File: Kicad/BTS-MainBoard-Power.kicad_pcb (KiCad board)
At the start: 2 copper layers, 101.6 x 95.3 mm, 47 parts, among them J1 +12VIn, J10 Conn_01x02, J11 Conn_01x02, J12 Conn_01x02, J13 Conn_01x02, J14 Conn_01x02, J15 Conn_01x02, J16 Conn_01x02, J17 Conn_01x02, J18 Conn_01x02, J19 Conn_01x02, J2 GNDIn, J3 Conn_01x14, J4 Conn_01x02, J5 Conn_01x02, J6 Conn_01x02, J7 Conn_01x02, J8 Conn_01x02, J9 Conn_01x02, Q1 STD80N6F6, Q2 STD80N6F6, Q3 STD80N6F6, Q4 STD80N6F6

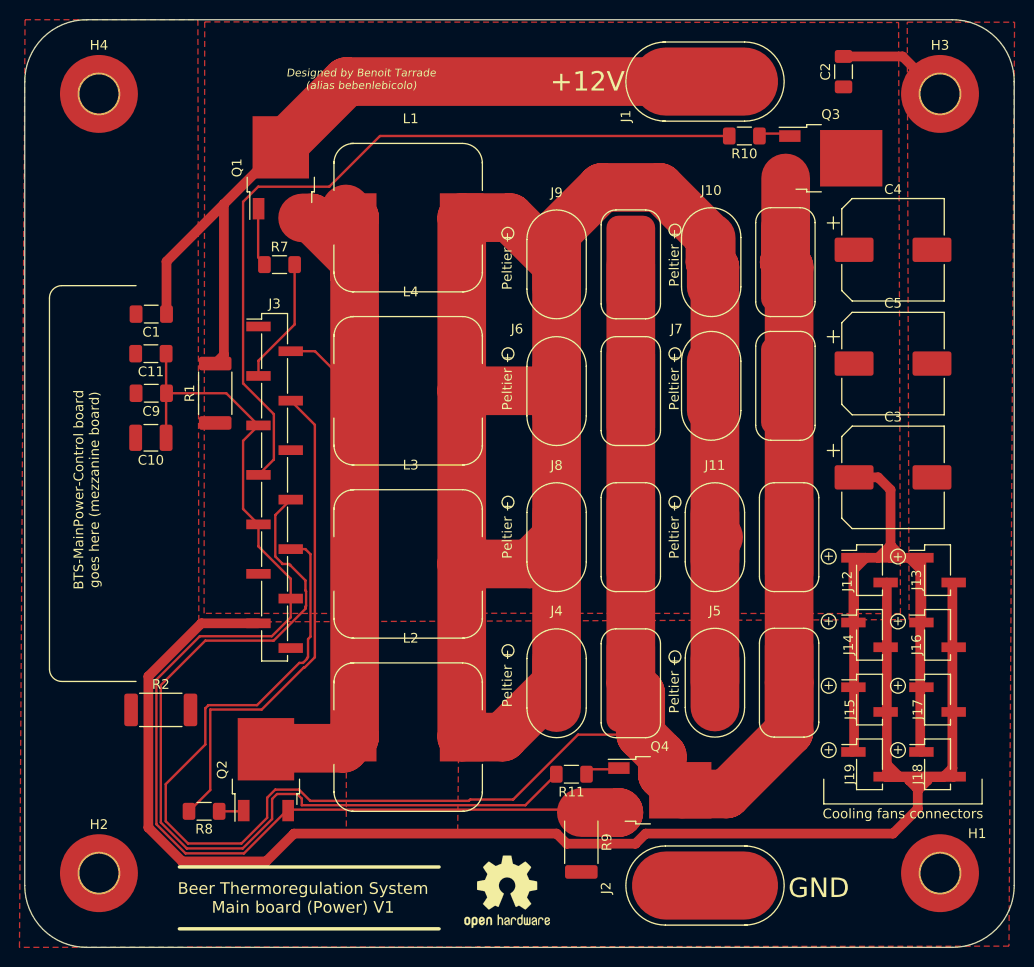
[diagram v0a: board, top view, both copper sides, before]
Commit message: Migrated kicad files to version 6
Signed-off-by: bebenlebricolo <benoittarrade@hotmail.fr>
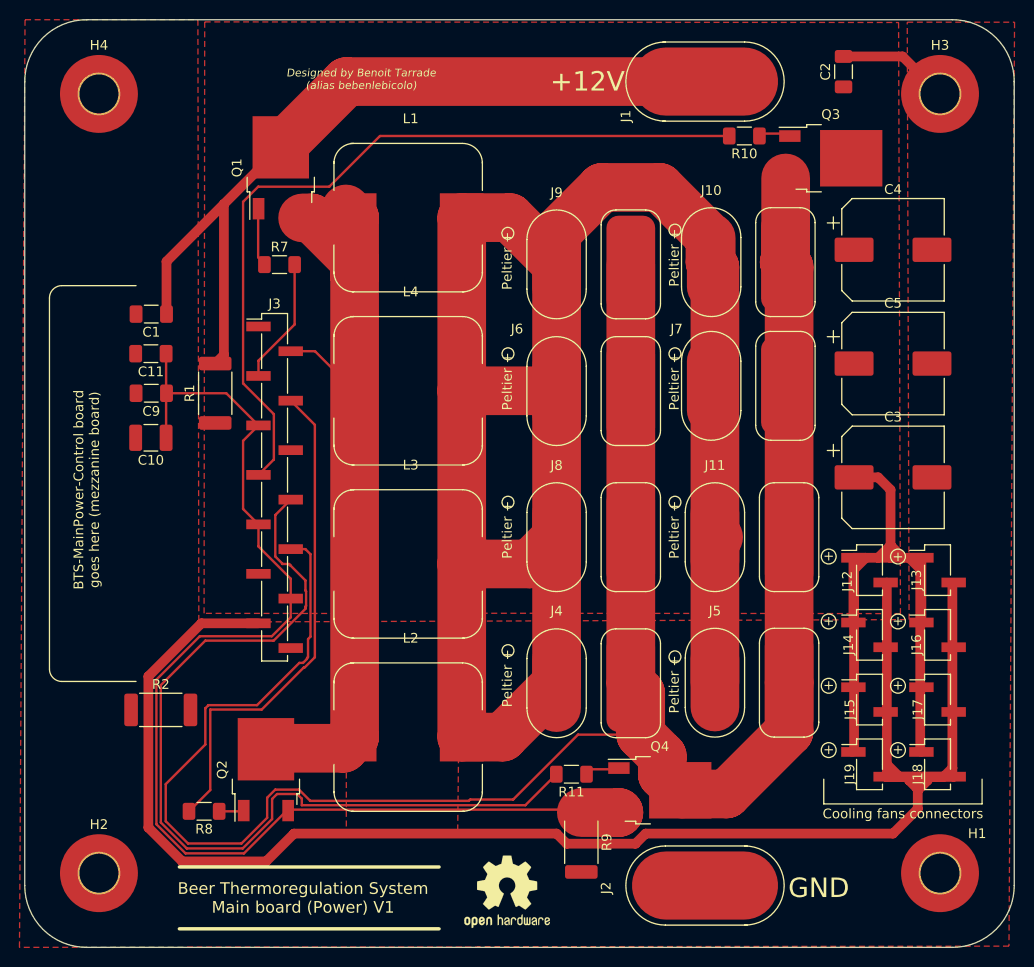
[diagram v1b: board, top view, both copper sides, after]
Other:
- board size 101.6 x 95.3 mm -> 101.6 x 95.2 mm
- net class Default removed
- net class Power track removed
